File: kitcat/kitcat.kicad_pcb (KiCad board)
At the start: 2 copper layers, 52 x 61.5 mm, 23 parts, among them IC1 LA4182, J1 Conn_01x02, J2 Conn_01x02, J3 Conn_01x02, J4 Conn_01x02, J5 Conn_01x02

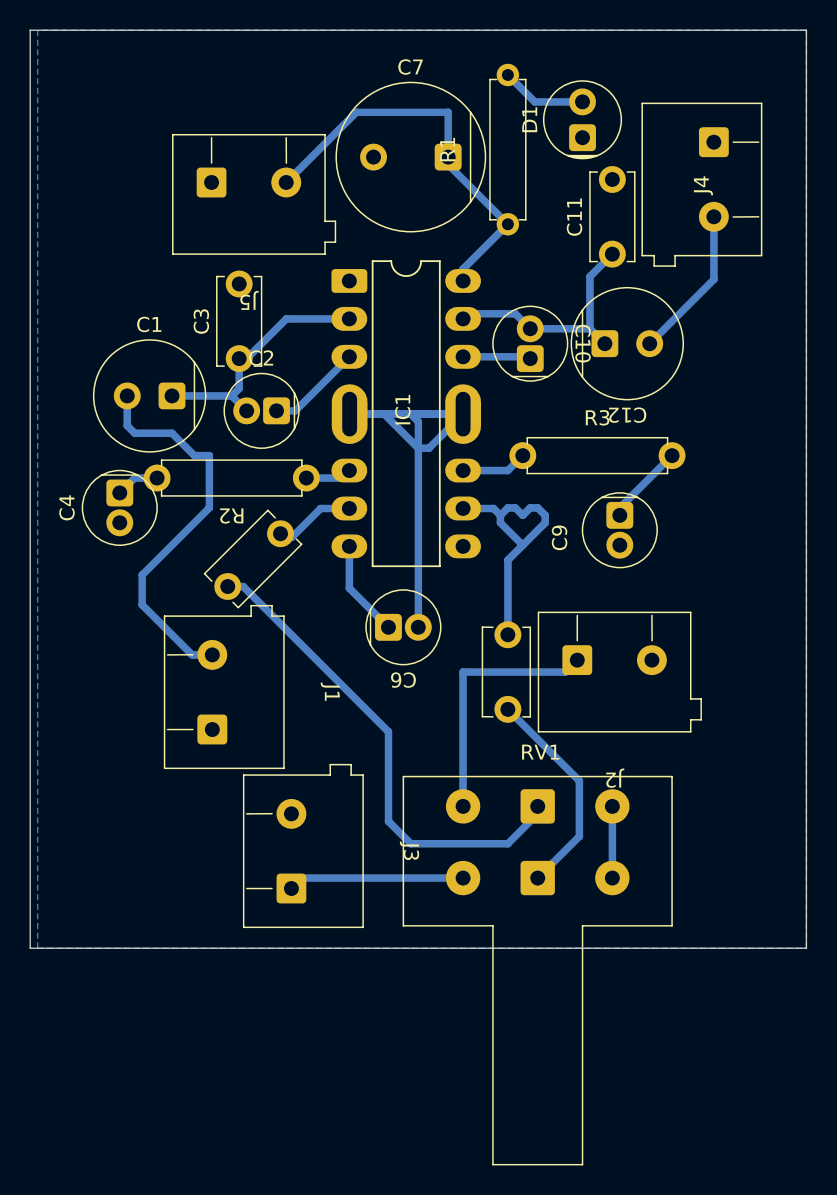
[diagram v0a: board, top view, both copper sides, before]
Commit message: hterhytnnnytjjyjnyt
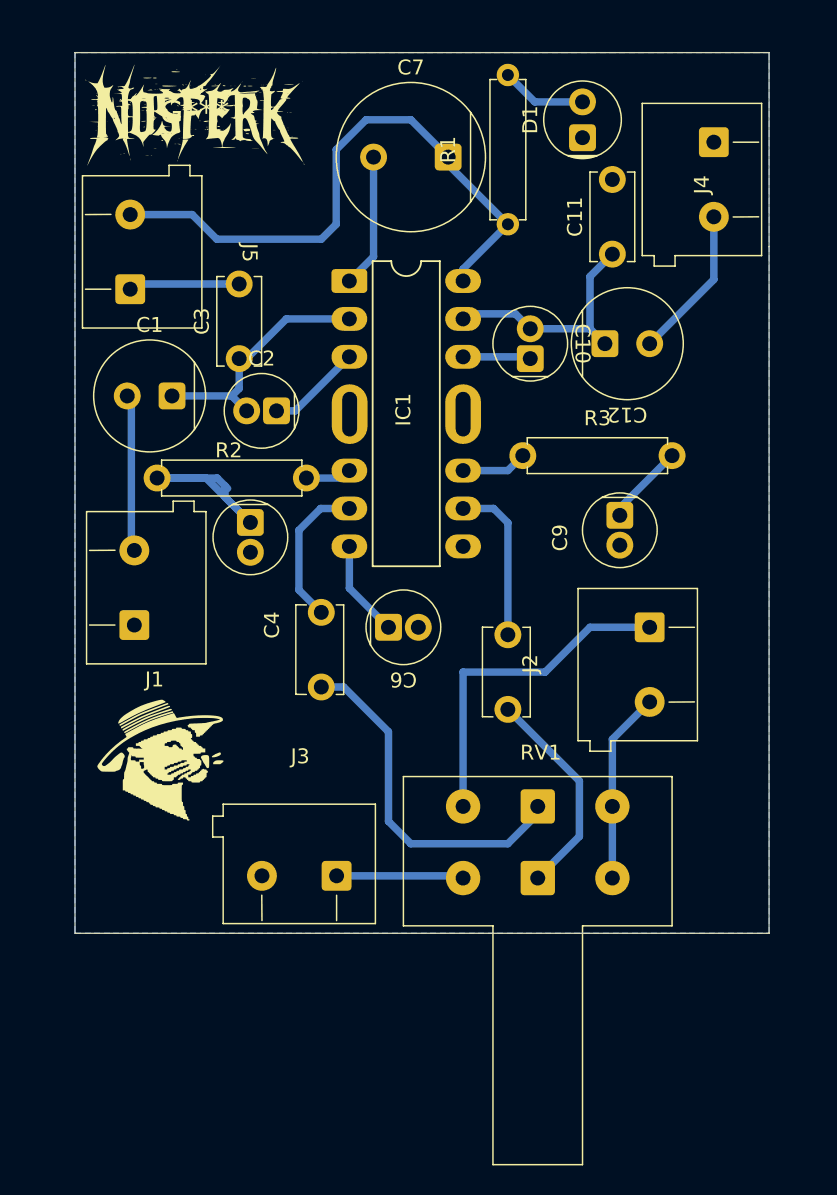
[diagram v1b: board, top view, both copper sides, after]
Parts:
- added G***: LOGO, LOGO, F.Cu at (156.2, 106.5)
- added G***: LOGO, LOGO, F.Cu at (158.5, 63.0)
- moved J5 9.21 mm to (154.2, 72.3), turned to -90 degrees
- moved C4 8.97 mm to (162.2, 91.5)
- moved J1 8.74 mm to (154.5, 94.8)
- moved C5 7.50 mm to (167.0, 99.0), turned to 90 degrees
- moved J2 2.37 mm to (189.0, 100.0), turned to 90 degrees
- moved J3 1.73 mm to (165.5, 114.2), turned to 0 degrees
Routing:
- net Net-(J1-Pin_1): track 26.3 -> 10.7 mm
- net GNDREF: track 44.0 -> 29.3 mm
- net Net-(IC1-12/VCC): track 27.0 -> 40.5 mm
- net Net-(C4-Pad1): track 2.91 -> 15.7 mm
- net Net-(C5-Pad1): track 32.7 -> 23.7 mm
- net Net-(IC1-8/IN1): track 18.2 -> 10.9 mm
- net Net-(J2-Pin_2): track 17.0 -> 22.7 mm
- net Net-(IC1-5/IN2): track 5.51 -> 10.1 mm
- net Net-(J3-Pin_2): track 11.8 -> 8.54 mm
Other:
- board size 52 x 61.5 mm -> 46.5 x 59 mm
